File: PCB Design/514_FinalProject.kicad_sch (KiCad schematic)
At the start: 13 parts, among them J1 Conn_01x04_Pin, J2 Conn_01x04_Pin, J3 Conn_01x04_Pin, J4 Conn_01x06_Pin, J5 Conn_01x02_Pin

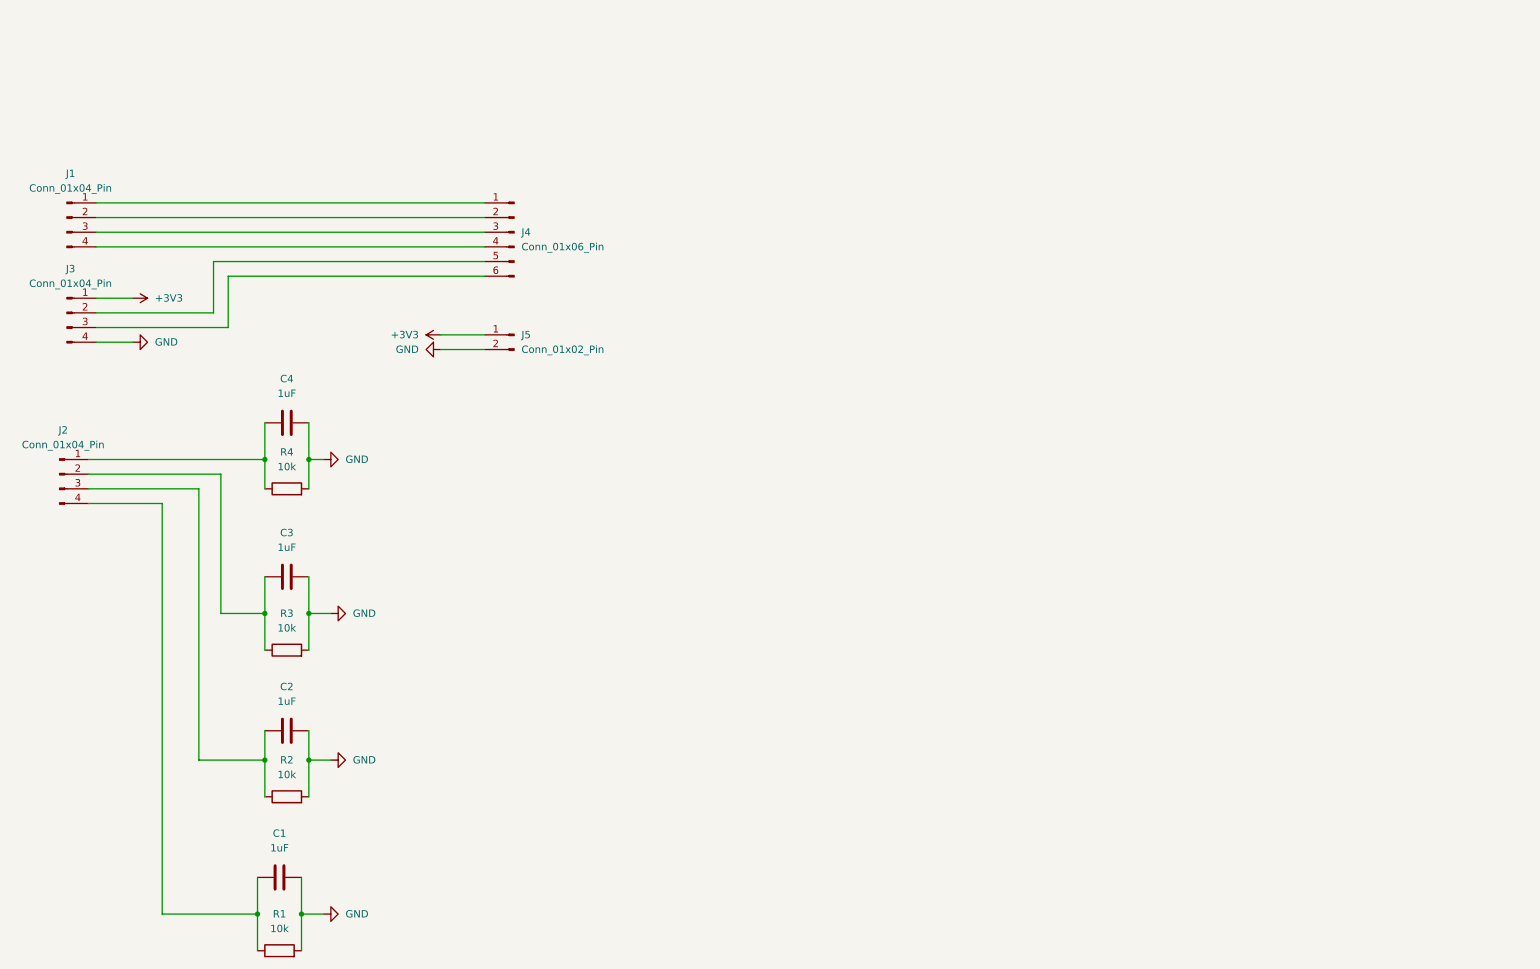
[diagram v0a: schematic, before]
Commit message: codes
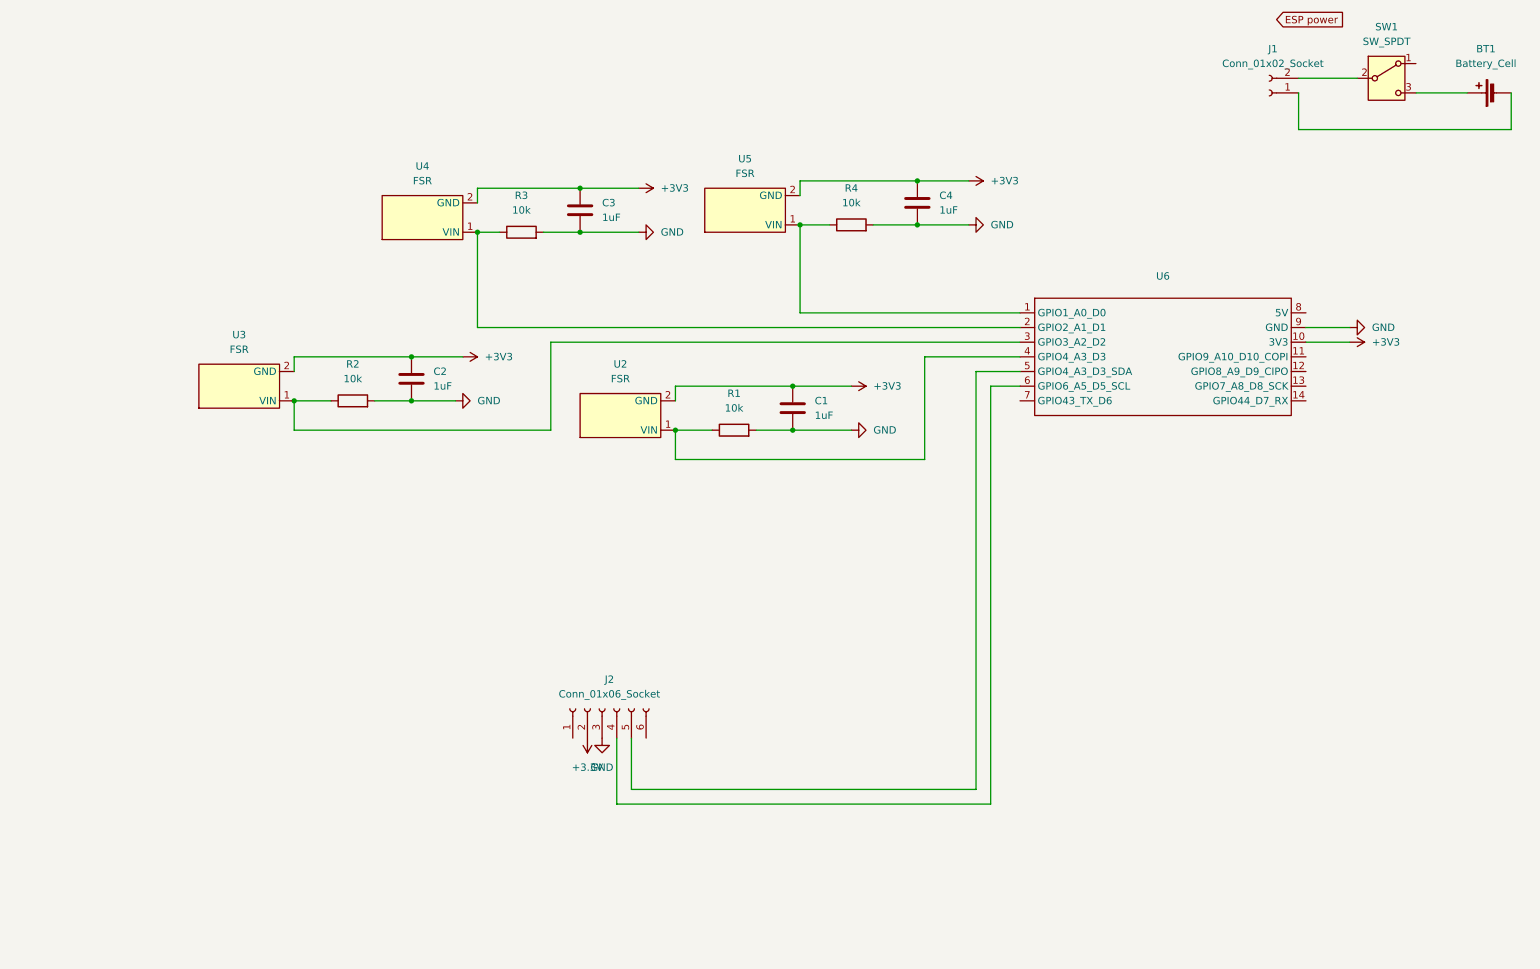
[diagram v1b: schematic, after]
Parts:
- removed J1, J2, J3: Conn_01x04_Pin, Connector_PinHeader_2.54mm:PinHeader_1x04_P2.54mm_Vertical, symbol Connector:Conn_01x04_Pin
- removed J4: Conn_01x06_Pin, Connector_PinHeader_2.54mm:PinHeader_1x06_P2.54mm_Vertical, symbol Connector:Conn_01x06_Pin
- removed J5: Conn_01x02_Pin, Connector_PinHeader_2.54mm:PinHeader_1x02_P2.54mm_Vertical, symbol Connector:Conn_01x02_Pin
- added BT1: Battery_Cell, Battery:BatteryHolder_Keystone_1042_1x18650, symbol Device:Battery_Cell
- added J1: Conn_01x02_Socket, Connector_PinHeader_2.54mm:PinHeader_1x02_P2.54mm_Vertical, symbol Connector:Conn_01x02_Socket
- added J2: Conn_01x06_Socket, Connector_PinHeader_2.54mm:PinHeader_1x05_P2.54mm_Vertical, symbol Connector:Conn_01x06_Socket
- added SW1: SW_SPDT, Connector_PinHeader_2.54mm:PinHeader_1x03_P2.54mm_Vertical, symbol Switch:SW_SPDT
- added U2, U3, U4, U5: FSR, Connector_PinHeader_2.54mm:PinHeader_1x02_P2.54mm_Vertical, symbol FSR:FSR
- added U6: ~, XIAO ESP32 S3:XIAO_ESP32_SENSE, symbol XIAO ESP 32 S3:XIAO_ESP32_SENSE
- C1: renamed from C4; footprint Capacitor_SMD:C_0402_1005Metric_Pad0.74x0.62mm_HandSolder -> Capacitor_SMD:C_0805_2012Metric_Pad1.18x1.45mm_HandSolder
- C2: renamed from C3; footprint Capacitor_SMD:C_0402_1005Metric_Pad0.74x0.62mm_HandSolder -> Capacitor_SMD:C_0805_2012Metric_Pad1.18x1.45mm_HandSolder
- C3: renamed from C2; footprint Capacitor_SMD:C_0402_1005Metric_Pad0.74x0.62mm_HandSolder -> Capacitor_SMD:C_0805_2012Metric_Pad1.18x1.45mm_HandSolder
- C4: renamed from C1; footprint Capacitor_SMD:C_0402_1005Metric_Pad0.74x0.62mm_HandSolder -> Capacitor_SMD:C_0805_2012Metric_Pad1.18x1.45mm_HandSolder
- R1: renamed from R4; footprint Resistor_SMD:R_0402_1005Metric_Pad0.72x0.64mm_HandSolder -> Resistor_SMD:R_0805_2012Metric_Pad1.20x1.40mm_HandSolder
- R2: renamed from R3; footprint Resistor_SMD:R_0402_1005Metric_Pad0.72x0.64mm_HandSolder -> Resistor_SMD:R_0805_2012Metric_Pad1.20x1.40mm_HandSolder
- R3: renamed from R2; footprint Resistor_SMD:R_0402_1005Metric_Pad0.72x0.64mm_HandSolder -> Resistor_SMD:R_0805_2012Metric_Pad1.20x1.40mm_HandSolder
- R4: renamed from R1; footprint Resistor_SMD:R_0402_1005Metric_Pad0.72x0.64mm_HandSolder -> Resistor_SMD:R_0805_2012Metric_Pad1.20x1.40mm_HandSolder
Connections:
- net +3V3: now also C1.1, C2.1, C3.1, C4.1, U2.2 (GND), U3.2 (GND), U4.2 (GND), U5.2 (GND), U6.10 (3V3)
- net GND: now also C1.2, C2.2, C3.2, C4.2, J2.3 (Pin_3), U6.9 (GND); no longer C1.1, C2.1, C3.1, C4.1
- net at R1.1: now also U2.1 (VIN), U6.4 (GPIO4_A3_D3); no longer C1.2
- net at R4.1: now also U5.1 (VIN), U6.1 (GPIO1_A0_D0); no longer C4.2
- net at R2.1: now also U3.1 (VIN), U6.3 (GPIO3_A2_D2); no longer C2.2
- net at R3.1: now also U4.1 (VIN), U6.2 (GPIO2_A1_D1); no longer C3.2
- new net: J1.2 (Pin_2), SW1.2 (B)
- new net: BT1.1 (+), SW1.3 (C)
- new net: BT1.2 (-), J1.1 (Pin_1)
- new net: J2.4 (Pin_4), U6.6 (GPIO6_A5_D5_SCL)
- new net: J2.5 (Pin_5), U6.5 (GPIO4_A3_D3_SDA)
- new net +3.3V: J2.2 (Pin_2)
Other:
- moved on the sheet: C1, C2, C3, C4, R1, R2, R3, R4
